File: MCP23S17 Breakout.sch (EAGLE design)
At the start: 10 parts, among them IC1 MCP23S17SO

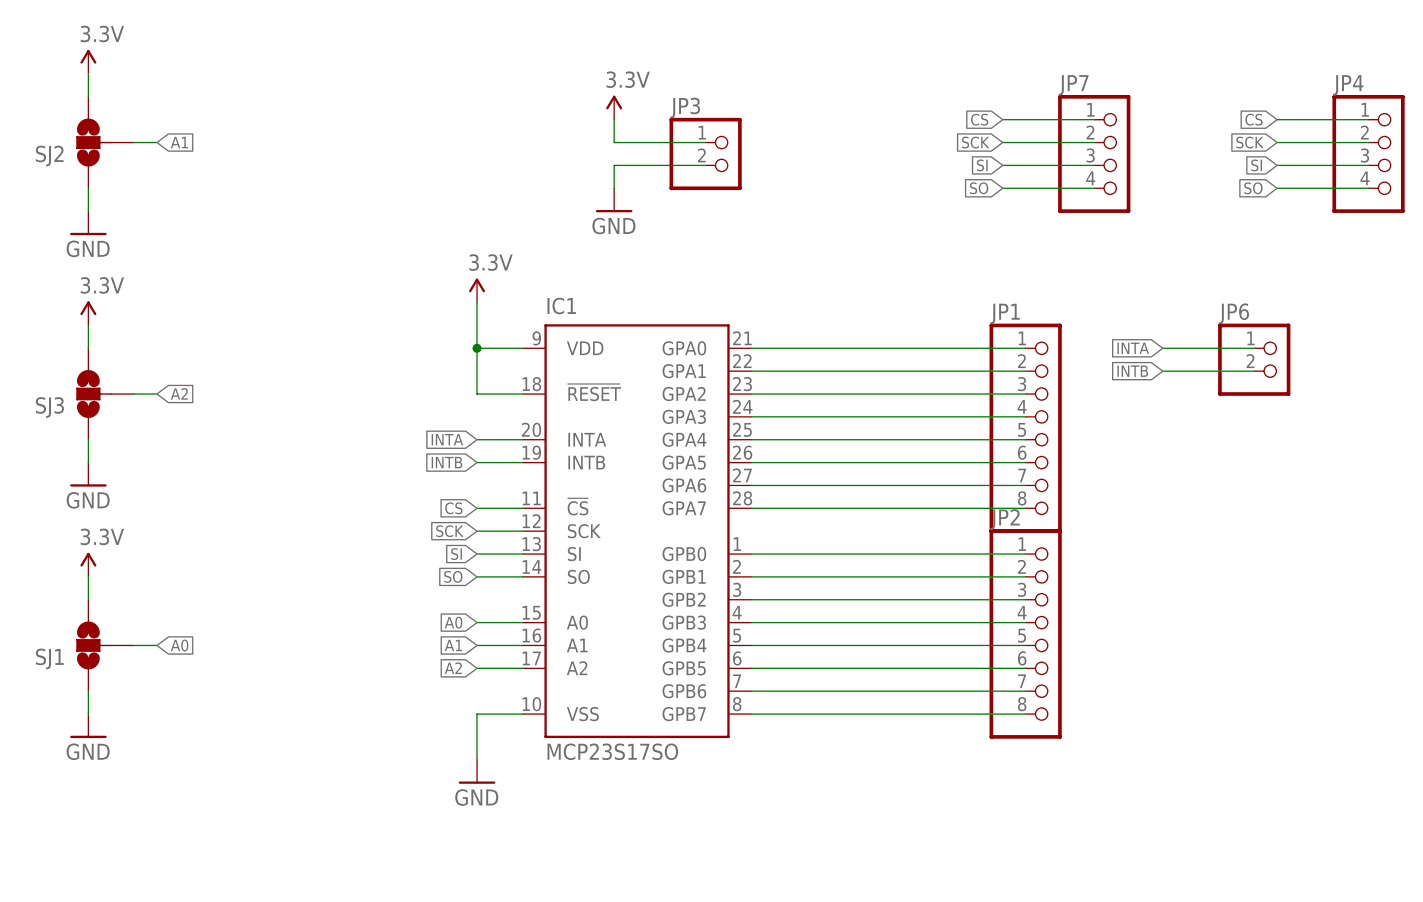
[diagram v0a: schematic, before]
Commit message: Update breakout
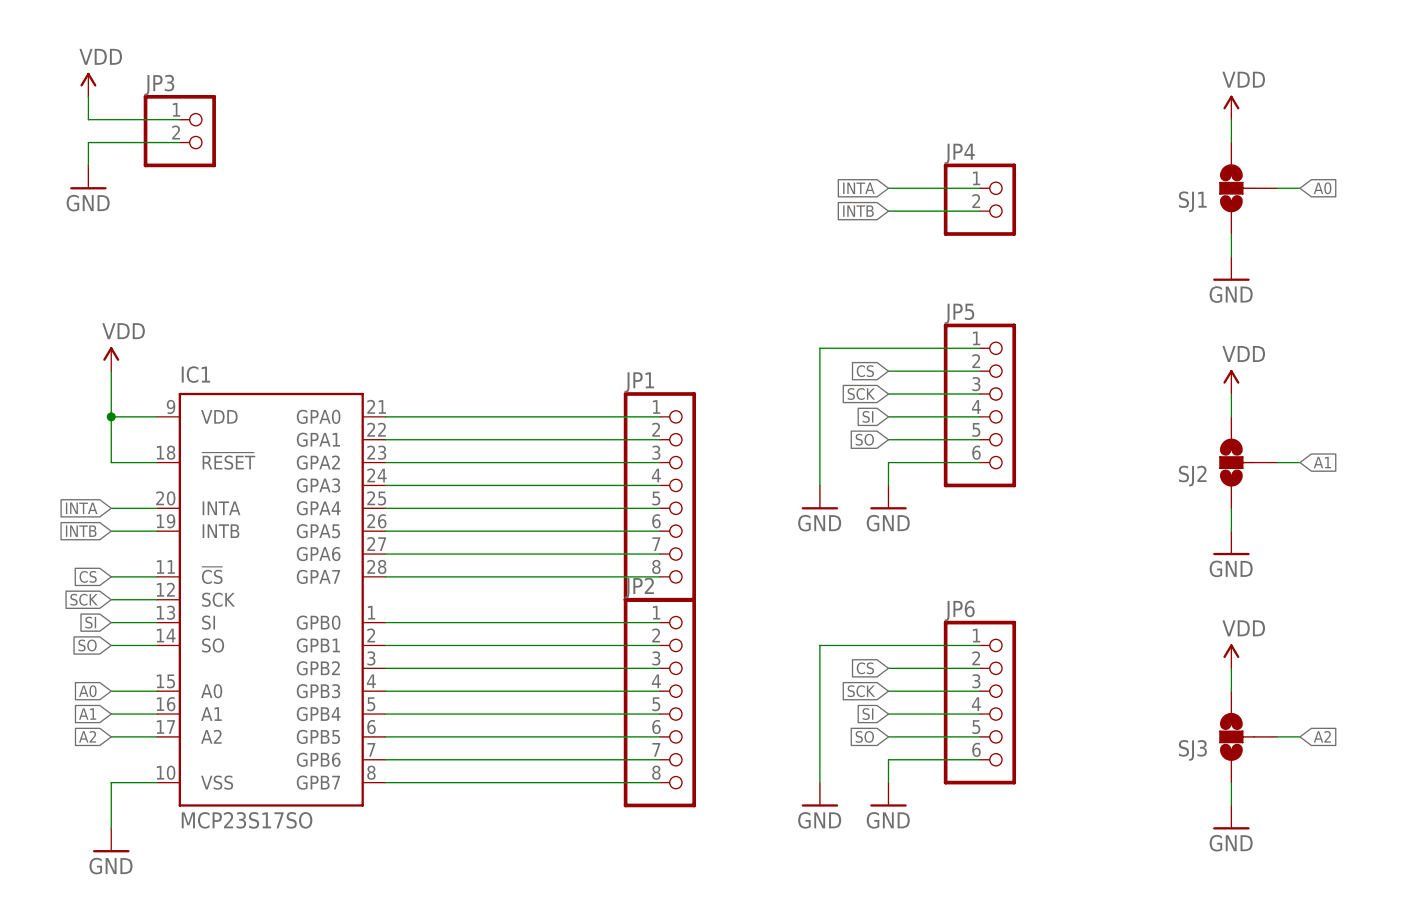
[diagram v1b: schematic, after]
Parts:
- removed JP7: (no value), pinhead:PINHD-1X4
- added JP5: (no value), pinhead:PINHD-1X6
- JP4: device pinhead:PINHD-1X4 -> pinhead:PINHD-1X2
- JP6: device pinhead:PINHD-1X2 -> pinhead:PINHD-1X6
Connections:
- net CS: now also JP5.2, JP6.2; no longer JP4.1, JP7.1
- net GND: now also JP5.1, JP5.6, JP6.1, JP6.6
- net INTA: now also JP4.1; no longer JP6.1
- net INTB: now also JP4.2; no longer JP6.2
- net SCK: now also JP5.3, JP6.3; no longer JP4.2, JP7.2
- net SI: now also JP5.4, JP6.4; no longer JP4.3, JP7.3
- net SO: now also JP5.5, JP6.5; no longer JP4.4, JP7.4
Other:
- moved on the sheet: IC1, JP1, JP2, JP3, SJ1, SJ2, SJ3
